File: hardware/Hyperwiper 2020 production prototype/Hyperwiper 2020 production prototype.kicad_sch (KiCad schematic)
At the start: 24 parts, among them J1 Conn_01x05, J2 USB_B, Q1 N-CH MOSFET, Q2 2N3904, SW1 SW_DPDT_x2, SW2 SW_Reed, U1 Teensy4.0, U3 Voltage regulator

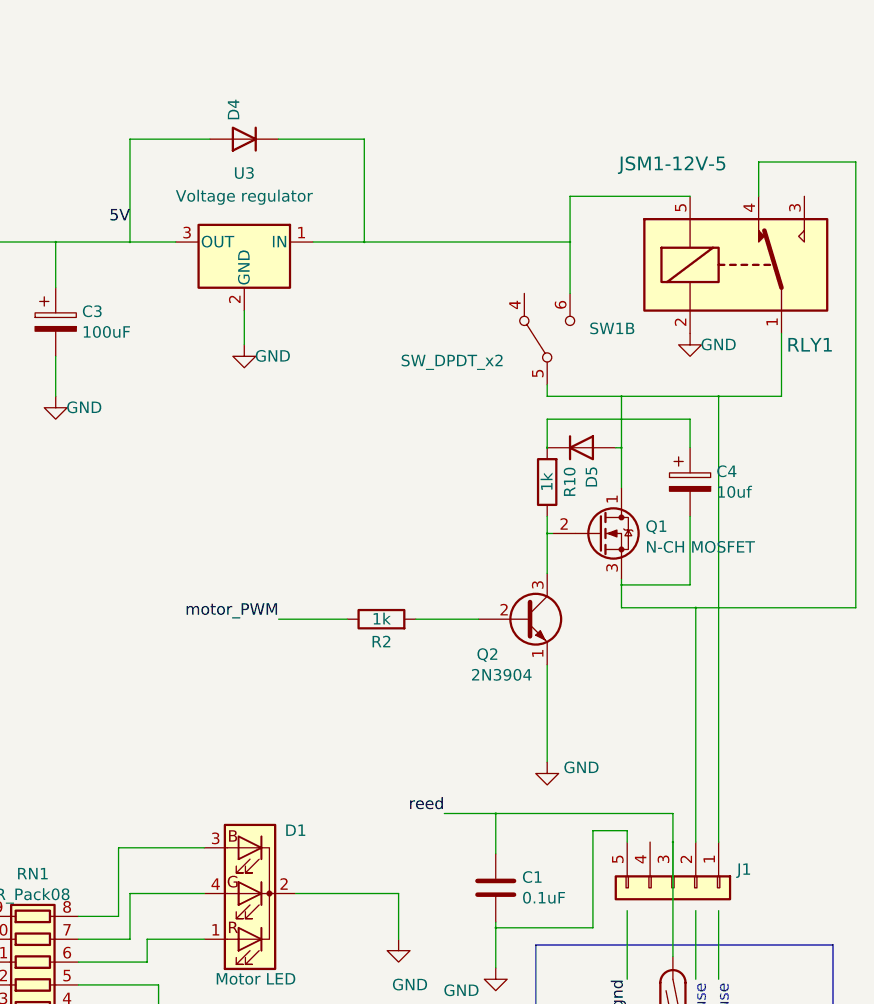
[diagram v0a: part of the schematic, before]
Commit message: Updates board
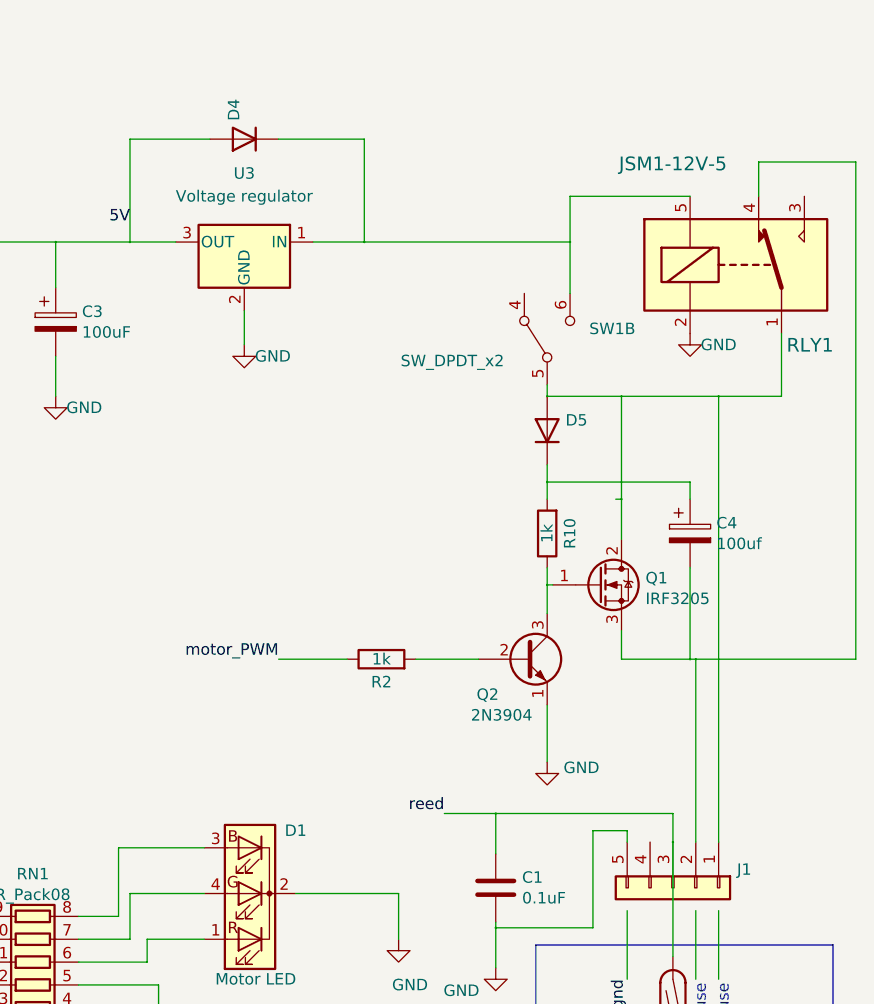
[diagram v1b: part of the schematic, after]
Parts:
- removed Q1: N-CH MOSFET, Package_DirectFET:DirectFET_MX, symbol Transistor_FET:BSB008NE2LX
- added Q1: IRF3205, Package_TO_SOT_THT:TO-220-3_Vertical, symbol Transistor_FET:IRF3205
- C4: value 10uf -> 100uf
- D5: value DIODE -> 1n4001
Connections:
- net at D5.1 (A), J1.1 (Pin_1), RLY1.1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: now also Q1.2 (D)
- net at C4.2, J1.2 (Pin_2), RLY1.4: now also Q1.3 (S)
- net at Q2.3 (C), R10.1: now also Q1.1 (G)
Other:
- moved on the sheet: C4, D5, Q2, R10, R2
